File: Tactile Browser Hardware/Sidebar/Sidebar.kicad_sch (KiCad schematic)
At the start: 0 parts

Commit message: I2C
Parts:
- added A1: Arduino_Nano_v3.x, Module:Arduino_Nano, symbol MCU_Module:Arduino_Nano_v3.x
- added Buck_converter: LM2596S-5, Package_TO_SOT_SMD:TO-263-5_TabPin3, symbol Regulator_Switching:LM2596S-5
- added R1, R2: R, symbol Device:R
- added SW1, SW2, SW3, SW4, SW5, SW6, SW7, SW8: SW_Push, symbol Switch:SW_Push
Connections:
- new net 5V: A1.27 (+5V)
- new net GND: A1.29 (GND), A1.4 (GND)
- new net SCL: A1.24 (A5)
- new net SDA: A1.23 (A4)

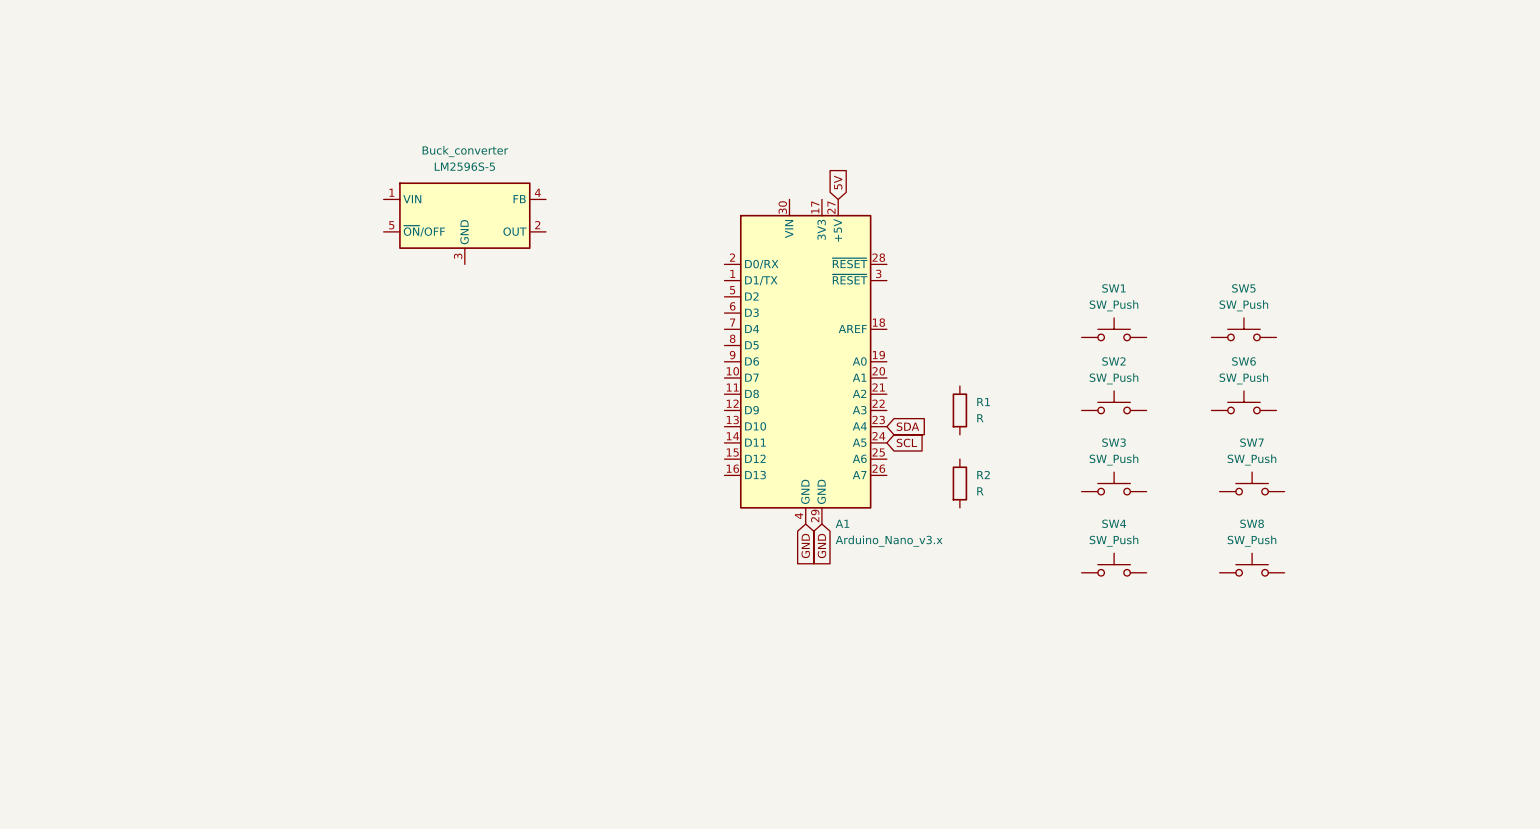
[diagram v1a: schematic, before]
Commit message: more sidebar progress
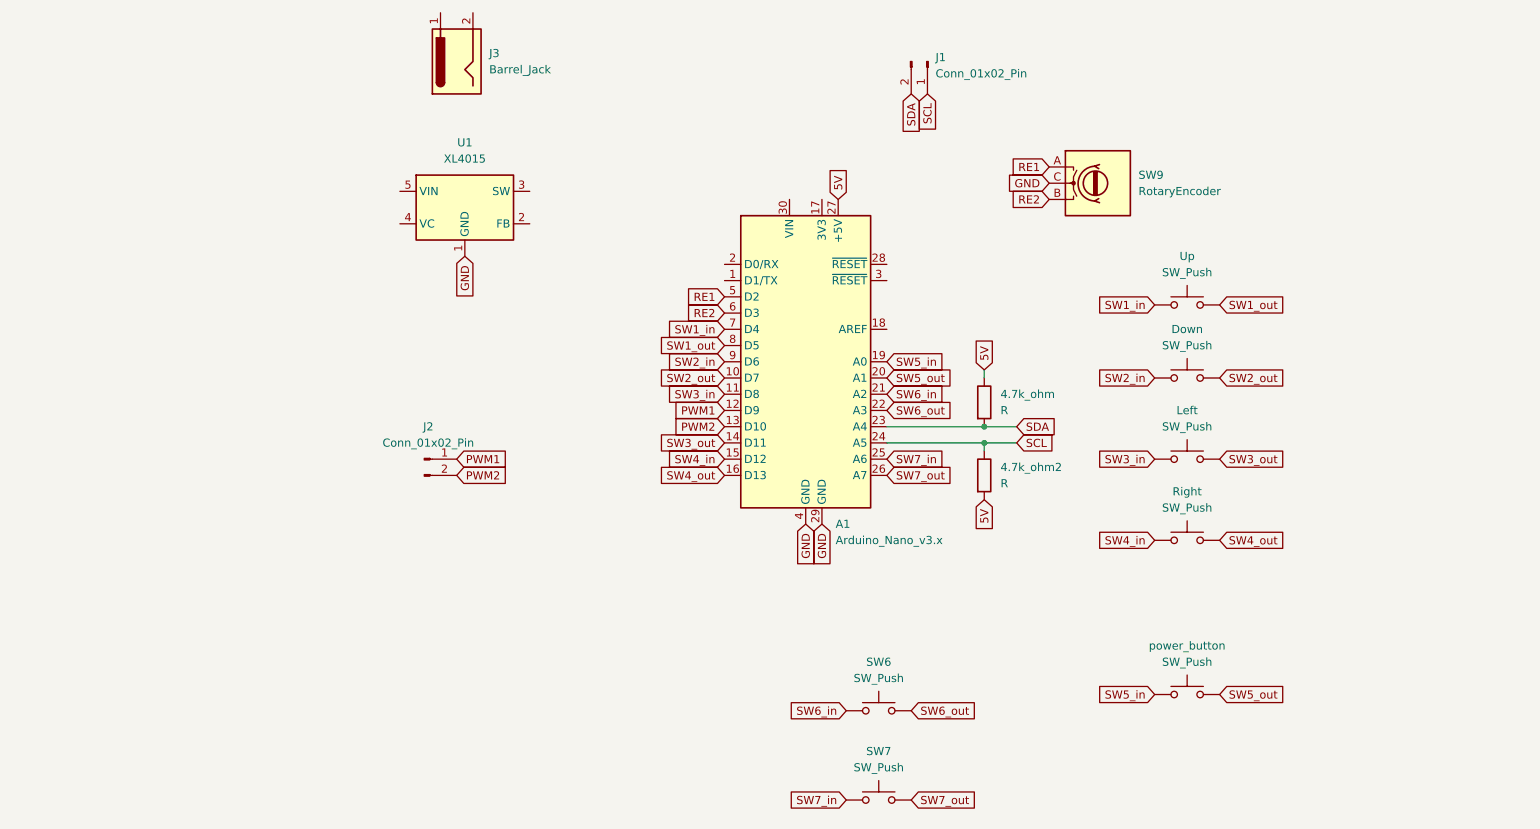
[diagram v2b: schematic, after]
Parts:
- removed Buck_converter: LM2596S-5, Package_TO_SOT_SMD:TO-263-5_TabPin3, symbol Regulator_Switching:LM2596S-5
- removed SW8: SW_Push, symbol Switch:SW_Push
- added J1, J2: Conn_01x02_Pin, symbol Connector:Conn_01x02_Pin
- added J3: Barrel_Jack, symbol Connector:Barrel_Jack
- added SW9: RotaryEncoder, symbol Device:RotaryEncoder
- added U1: XL4015, Package_TO_SOT_SMD:TO-263-5_TabPin3, symbol Regulator_Switching:XL4015
- renumbered R1 to 4.7k_ohm, R2 to 4.7k_ohm2, SW2 to Down, SW3 to Left, SW4 to Right, SW1 to Up, SW5 to power_button
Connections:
- net 5V: now also 4.7k_ohm.1, 4.7k_ohm2.2
- net GND: now also SW9.C, U1.1 (GND)
- net SCL: now also 4.7k_ohm2.1, J1.1 (Pin_1)
- net SDA: now also 4.7k_ohm.2, J1.2 (Pin_2)
- net SW5_in: now reaches power_button.1
- net SW5_in: now also A1.19 (A0)
- net SW5_out: now reaches power_button.2
- net SW5_out: now also A1.20 (A1)
- net SW6_in: now reaches SW6.1
- net SW6_in: now also A1.21 (A2)
- net SW6_out: now reaches SW6.2
- net SW6_out: now also A1.22 (A3)
- net SW3_in: now reaches Left.1
- net SW3_in: now also A1.11 (D8)
- net SW3_out: now reaches Left.2
- net SW3_out: now also A1.14 (D11)
- net SW2_out: now reaches A1.10 (D7)
- net SW2_out: now also Down.2
- net PWM1: now reaches A1.12 (D9)
- net PWM1: now also J2.1 (Pin_1)
- net PWM2: now reaches A1.13 (D10)
- net PWM2: now also J2.2 (Pin_2)
- net SW4_in: now reaches A1.15 (D12)
- net SW4_in: now also Right.1
- net SW4_out: now reaches A1.16 (D13)
- net SW4_out: now also Right.2
- net SW7_in: now reaches A1.25 (A6)
- net SW7_in: now also SW7.1
- net SW7_out: now reaches A1.26 (A7)
- net SW7_out: now also SW7.2
- net RE1: now reaches A1.5 (D2)
- net RE1: now also SW9.A
- net RE2: now reaches A1.6 (D3)
- net RE2: now also SW9.B
- net SW1_in: now reaches A1.7 (D4)
- net SW1_in: now also Up.1
- net SW1_out: now reaches A1.8 (D5)
- net SW1_out: now also Up.2
- net SW2_in: now reaches A1.9 (D6)
- net SW2_in: now also Down.1
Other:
- moved on the sheet: 4.7k_ohm, 4.7k_ohm2, Down, Left, Right, SW6, SW7, Up, power_button

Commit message: sidebar progress
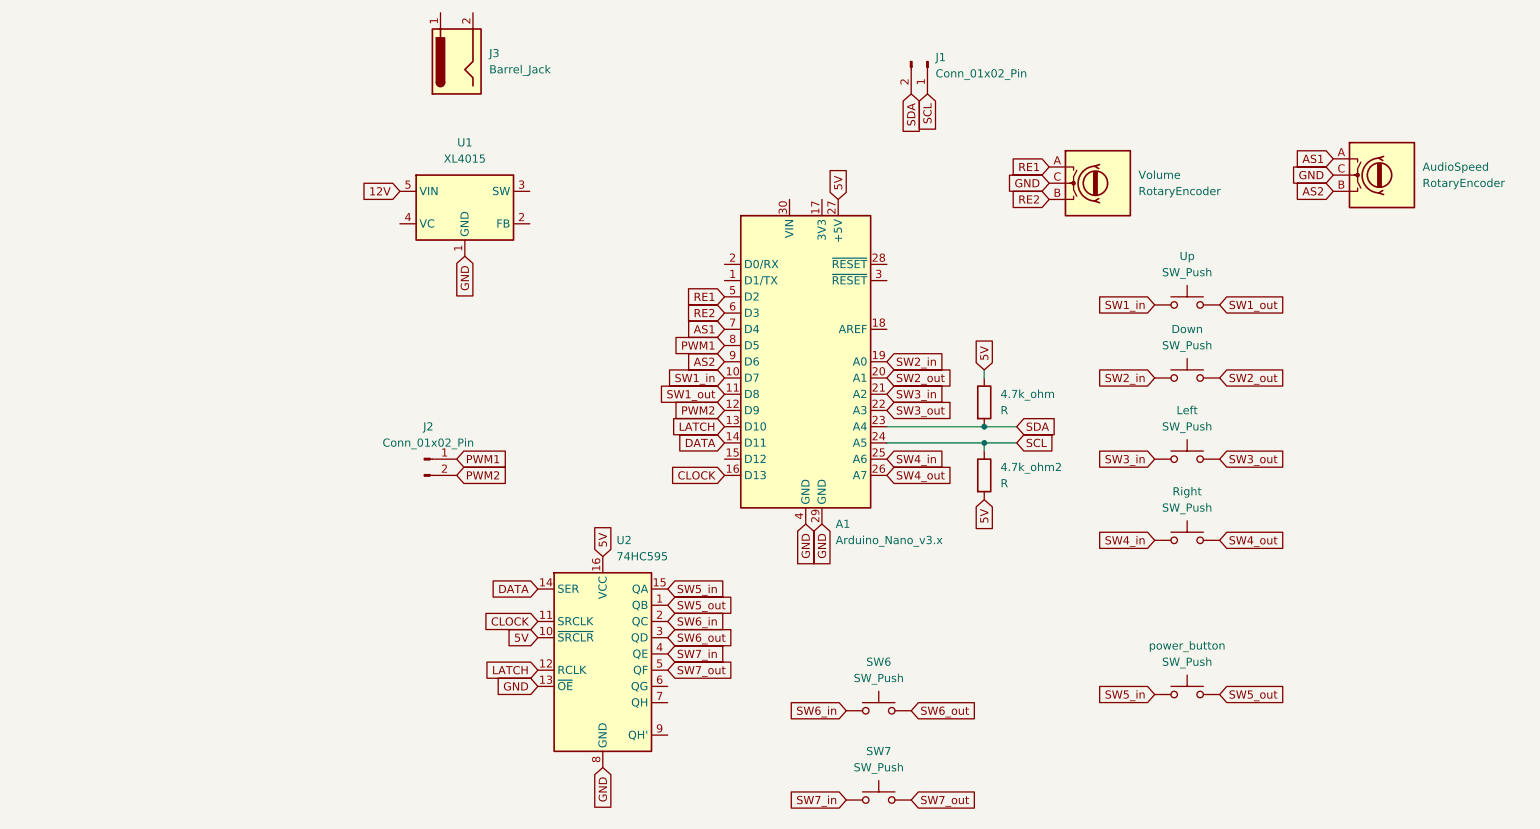
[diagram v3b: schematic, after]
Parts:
- added AudioSpeed: RotaryEncoder, symbol Device:RotaryEncoder
- added U2: 74HC595, symbol 74xx:74HC595
- renumbered SW9 to Volume
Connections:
- net 5V: now also U2.10 (~{SRCLR}), U2.16 (VCC)
- net GND: now also AudioSpeed.C, U2.13 (~{OE}), U2.8 (GND)
- net PWM1: now also A1.8 (D5); no longer A1.12 (D9)
- net PWM2: now also A1.12 (D9); no longer A1.13 (D10)
- net SW1_in: now also A1.10 (D7); no longer A1.7 (D4)
- net SW1_out: now also A1.11 (D8); no longer A1.8 (D5)
- net SW2_in: now also A1.19 (A0); no longer A1.9 (D6)
- net SW2_out: now also A1.20 (A1); no longer A1.10 (D7)
- net SW3_in: now also A1.21 (A2); no longer A1.11 (D8)
- net SW3_out: now also A1.22 (A3); no longer A1.14 (D11)
- net SW4_in: now also A1.25 (A6); no longer A1.15 (D12)
- net SW4_out: now also A1.26 (A7); no longer A1.16 (D13)
- net SW5_in: now also U2.15 (QA); no longer A1.19 (A0)
- net SW5_out: now also U2.1 (QB); no longer A1.20 (A1)
- net SW6_in: now also U2.2 (QC); no longer A1.21 (A2)
- net SW6_out: now also U2.3 (QD); no longer A1.22 (A3)
- net SW7_in: now also U2.4 (QE); no longer A1.25 (A6)
- net SW7_out: now also U2.5 (QF); no longer A1.26 (A7)
- net 12V: now reaches U1.5 (VIN)
- new net AS1: A1.7 (D4), AudioSpeed.A
- new net AS2: A1.9 (D6), AudioSpeed.B
- new net CLOCK: A1.16 (D13), U2.11 (SRCLK)
- new net DATA: A1.14 (D11), U2.14 (SER)
- new net LATCH: A1.13 (D10), U2.12 (RCLK)

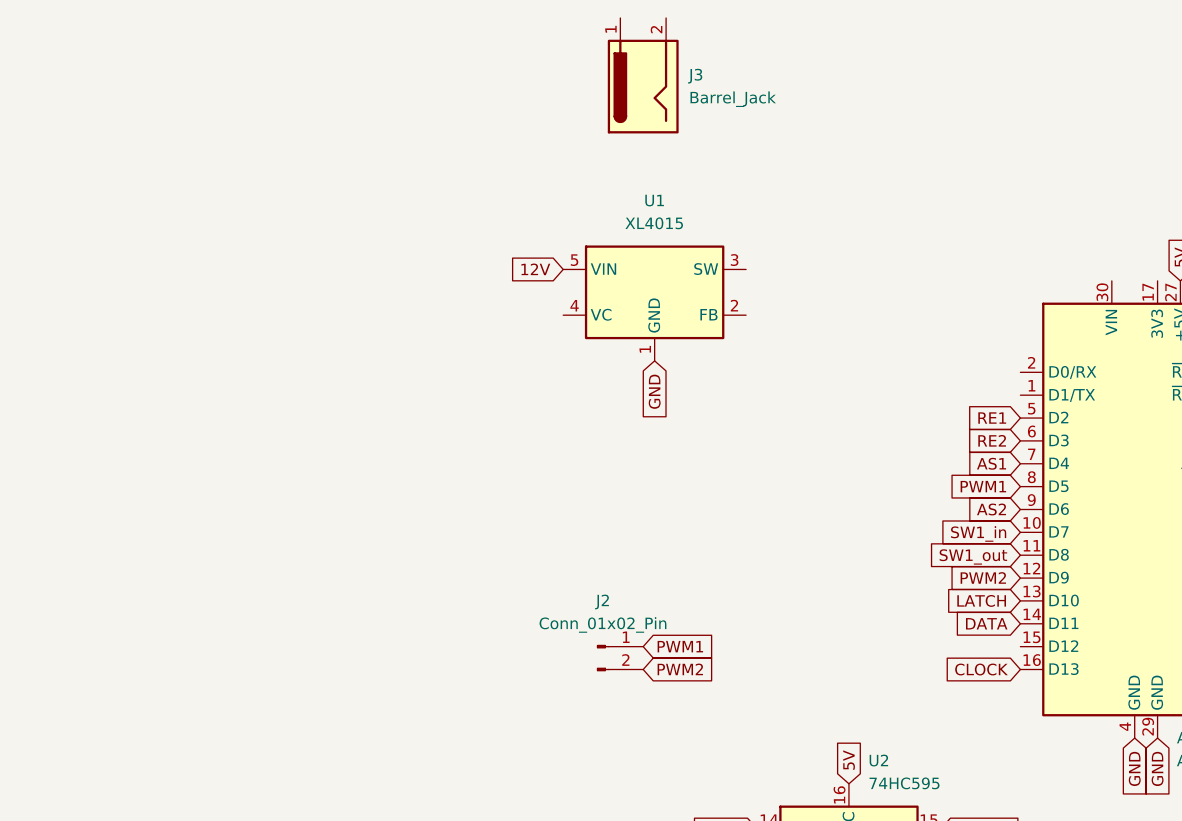
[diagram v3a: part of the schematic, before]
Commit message: electrical safety
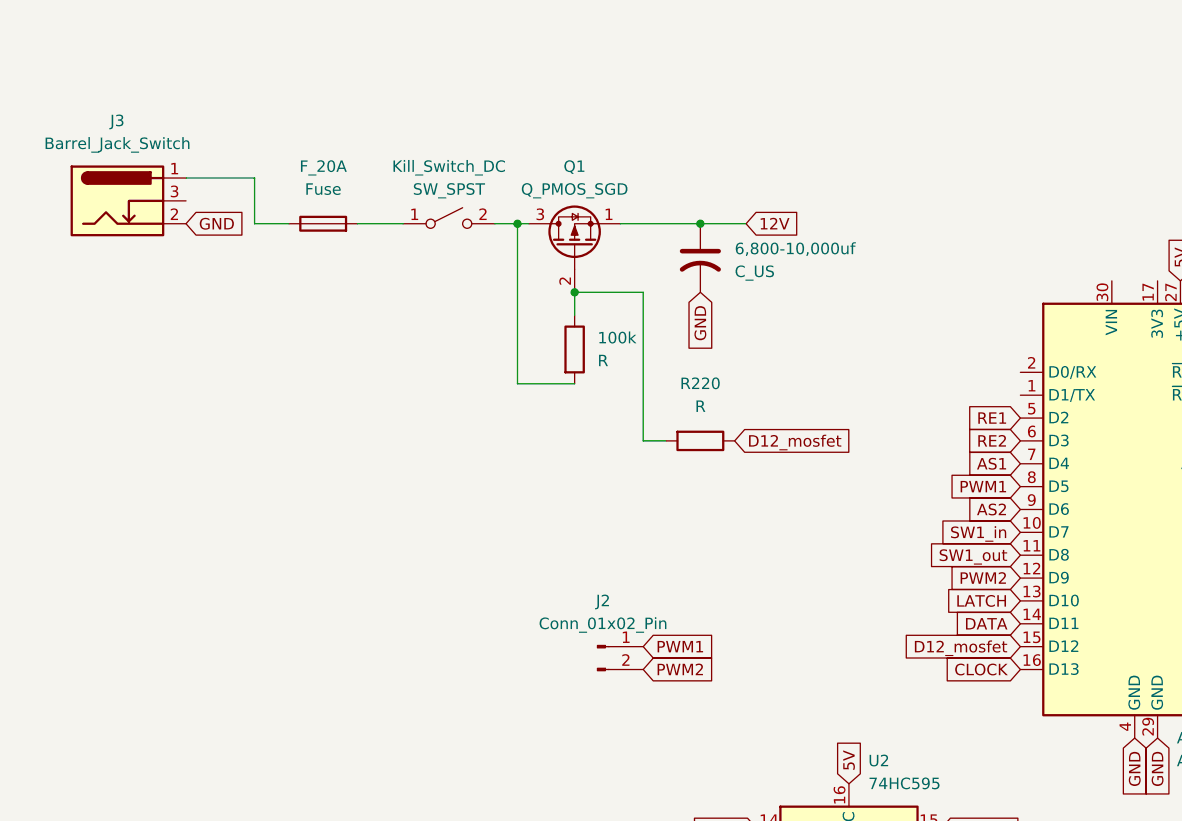
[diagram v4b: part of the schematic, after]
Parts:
- removed J3: Barrel_Jack, symbol Connector:Barrel_Jack
- removed U1: XL4015, Package_TO_SOT_SMD:TO-263-5_TabPin3, symbol Regulator_Switching:XL4015
- added 100k, R220: R, symbol Device:R
- added 6,800-10,000uf: C_US, symbol Device:C_US
- added F_20A: Fuse, symbol Device:Fuse
- added J3: Barrel_Jack_Switch, symbol Connector:Barrel_Jack_Switch
- added Kill_Switch_DC: SW_SPST, symbol Switch:SW_SPST
- added Q1: Q_PMOS_SGD, symbol Transistor_FET:Q_PMOS_SGD
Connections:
- net 12V: now also 6,800-10,000uf.1, Q1.1 (S)
- net GND: now also 6,800-10,000uf.2, J3.2
- net D12_mosfet: now reaches A1.15 (D12)
- net D12_mosfet: now also R220.1
- new net: 100k.1, Q1.2 (G), R220.2
- new net: 100k.2, Kill_Switch_DC.2 (B), Q1.3 (D)
- new net: F_20A.1, J3.1
- new net: F_20A.2, Kill_Switch_DC.1 (A)
